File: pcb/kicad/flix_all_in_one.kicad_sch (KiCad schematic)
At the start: 0 parts

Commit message: Updated sch and added BoM.md
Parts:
- added U1: ESP32-WROOM-32E, RF_Module:ESP32-WROOM-32E, symbol RF_Module:ESP32-WROOM-32E
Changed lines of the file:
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@@
 	(generator_version "10.0")
 	(paper "A4")
+	(symbol
+		(lib_id "RF_Module:ESP32-WROOM-32E")
+		(at 148.59 102.87 0)
+		(unit 1)
+		(body_style 1)
+		(exclude_from_sim no)
+		(in_bom yes)
+		(on_board yes)
+		(in_pos_files yes)
+		(dnp no)
+		(fields_autoplaced yes)
+		(property "Reference" "U1"
+			(at 150.7333 64.77 0)
+			(show_name no)
+			(do_not_autoplace no)
+			(effects
+				(font
+					(size 1.27 1.27)
+				)
+				(justify left)
+			)
+		)
+		(property "Value" "ESP32-WROOM-32E"
+			(at 150.7333 67.31 0)
+			(show_name no)
+			(do_not_autoplace no)
+			(effects
+				(font
+					(size 1.27 1.27)
+				)
+				(justify left)
+			)
+		)
+		(property "Footprint" "RF_Module:ESP32-WROOM-32E"
+			(at 165.1 137.16 0)
+			(hide yes)
+			(show_name no)
+			(do_not_autoplace no)
+			(effects
+				(font
+					(size 1.27 1.27)
+				)
+			)
+		)
+		(property "Datasheet" "https://www.espressif.com/sites/default/files/documentation/esp32-wroom-32e_esp32-wroom-32ue_datasheet_en.pdf"
+			(at 148.59 102.87 0)
+			(hide yes)
+			(show_name no)
+			(do_not_autoplace no)
+			(effects
+				(font
+					(size 1.27 1.27)
+				)
+			)
+		)
+		(property "Description" "RF Module, ESP32-D0WD-V3 SoC, without PSRAM, Wi-Fi 802.11b/g/n, Bluetooth, BLE, 32-bit, 2.7-3.6V, onboard antenna, SMD"
+			(at 148.59 102.87 0)
+			(hide yes)
+			(show_name no)
+			(do_not_autoplace no)
+			(effects
+				(font
+					(size 1.27 1.27)
+				)
+			)
+		)
+		(pin "14"
+		)
+		(pin "11"
+		)
+		(pin "16"
+		)
+		(pin "12"
+		)
+		(pin "9"
+		)
+		(pin "17"
+		)
+		(pin "13"
+		)
+		(pin "30"
+		)
+		(pin "33"
+		)
+		(pin "27"
+		)
+		(pin "31"
+		)
+		(pin "10"
+		)
+		(pin "32"
+		)
+		(pin "34"
+		)
+		(pin "18"
+		)
+		(pin "26"
+		)
+		(pin "28"
+		)
+		(pin "19"
+		)
+		(pin "21"
+		)
+		(pin "35"
+		)
+		(pin "36"
+		)
+		(pin "29"
+		)
+		(pin "[1,15,38,39]"
+		)
+		(pin "3"
+		)
+		(pin "2"
+		)
+		(pin "20"
+		)
+		(pin "4"
+		)
+		(pin "25"
+		)
+		(pin "6"
+		)
+		(pin "24"
+		)
+		(pin "5"
+		)
+		(pin "7"
+		)
+		(pin "8"
+		)
+		(pin "37"
+		)
+		(pin "22"
+		)
+		(pin "23"
+		)
+		(instances
+			(project "flix_all_in_one"
+				(path "/b72e5080-03e0-4f53-a508-ed803e54cf11"
+					(reference "U1")
+					(unit 1)
+				)
+			)
+		)
+	)
 	(sheet_instances
 		(path "/"

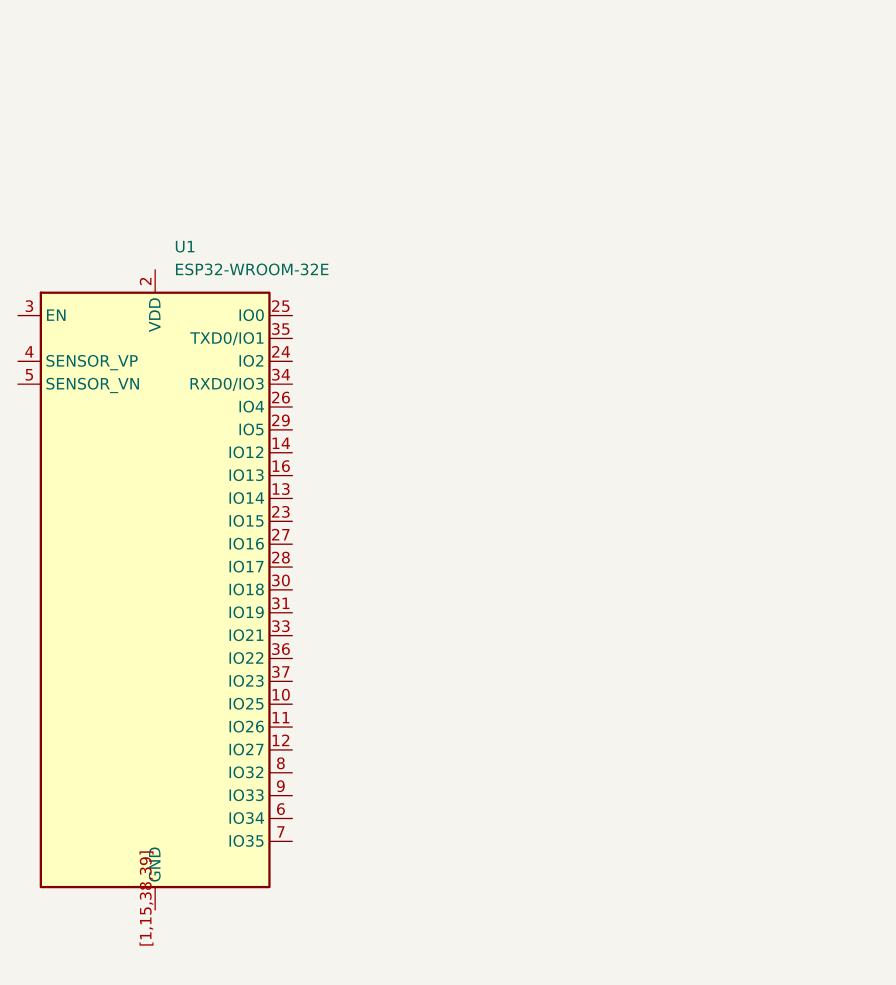
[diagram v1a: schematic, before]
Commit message: .
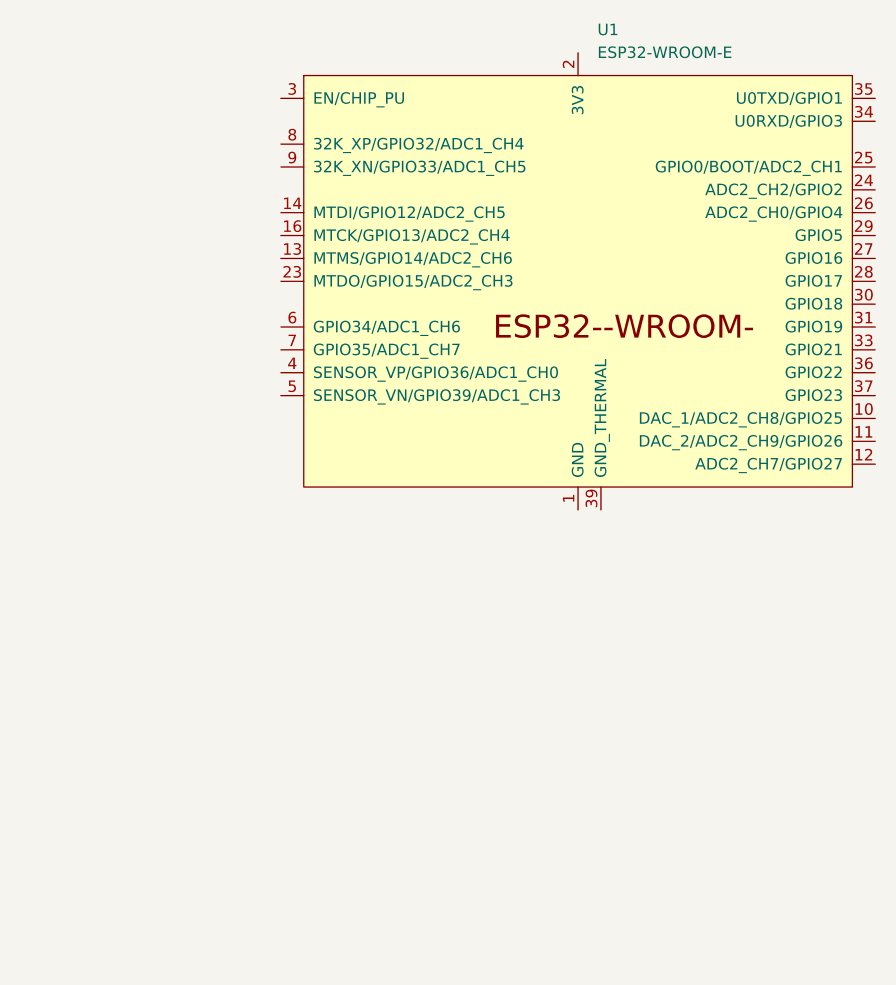
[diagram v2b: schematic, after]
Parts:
- removed U1: ESP32-WROOM-32E, RF_Module:ESP32-WROOM-32E, symbol RF_Module:ESP32-WROOM-32E
- added U1: ESP32-WROOM-E, PCM_Espressif:ESP32-WROOM-32E, symbol PCM_Espressif:ESP32-WROOM-E
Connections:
- new net: U1.1 (GND), U1.15 (GND), U1.38 (GND)
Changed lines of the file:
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@@
 	(paper "A4")
 	(symbol
-		(lib_id "RF_Module:ESP32-WROOM-32E")
-		(at 148.59 102.87 0)
+		(lib_id "PCM_Espressif:ESP32-WROOM-E")
+		(at 195.58 68.58 0)
 		(unit 1)
 		(body_style 1)
@@
 		(fields_autoplaced yes)
 		(property "Reference" "U1"
-			(at 150.7333 64.77 0)
+			(at 197.7233 40.64 0)
 			(show_name no)
 			(do_not_autoplace no)
@@
 			)
 		)
-		(property "Value" "ESP32-WROOM-32E"
-			(at 150.7333 67.31 0)
+		(property "Value" "ESP32-WROOM-E"
+			(at 197.7233 43.18 0)
 			(show_name no)
 			(do_not_autoplace no)
@@
 			)
 		)
-		(property "Footprint" "RF_Module:ESP32-WROOM-32E"
-			(at 165.1 137.16 0)
+		(property "Footprint" "PCM_Espressif:ESP32-WROOM-32E"
+			(at 195.58 104.14 0)
 			(hide yes)
 			(show_name no)
@@
 		)
 		(property "Datasheet" "https://www.espressif.com/sites/default/files/documentation/esp32-wroom-32e_esp32-wroom-32ue_datasheet_en.pdf"
-			(at 148.59 102.87 0)
+			(at 195.58 106.68 0)
 			(hide yes)
 			(show_name no)
@@
 			)
 		)
-		(property "Description" "RF Module, ESP32-D0WD-V3 SoC, without PSRAM, Wi-Fi 802.11b/g/n, Bluetooth, BLE, 32-bit, 2.7-3.6V, onboard antenna, SMD"
-			(at 148.59 102.87 0)
+		(property "Description" "ESP32-WROOM-32E integrates ESP32-D0WD-V3, with higher stability and safety performance."
+			(at 195.58 68.58 0)
 			(hide yes)
 			(show_name no)
@@
 			)
 		)
-		(pin "14"
+		(pin "15"
 		)
-		(pin "11"
+		(pin "30"
 		)
-		(pin "16"
-		)
-		(pin "12"
-		)
-		(pin "9"
-		)
-		(pin "17"
+		(pin "31"
 		)
 		(pin "13"
 		)
-		(pin "30"
-		)
-		(pin "33"
-		)
-		(pin "27"
-		)
-		(pin "31"
-		)
-		(pin "10"
-		)
-		(pin "32"
-		)
-		(pin "34"
-		)
-		(pin "18"
-		)
-		(pin "26"
-		)
-		(pin "28"
-		)
-		(pin "19"
-		)
-		(pin "21"
+		(pin "25"
 		)
 		(pin "35"
@@
 		(pin "36"
 		)
+		(pin "33"
+		)
 		(pin "29"
 		)
-		(pin "[1,15,38,39]"
+		(pin "34"
+		)
+		(pin "37"
+		)
+		(pin "14"
+		)
+		(pin "7"
+		)
+		(pin "26"
+		)
+		(pin "9"
+		)
+		(pin "27"
+		)
+		(pin "5"
+		)
+		(pin "4"
 		)
 		(pin "3"
 		)
-		(pin "2"
+		(pin "23"
 		)
-		(pin "20"
+		(pin "39"
 		)
-		(pin "4"
+		(pin "12"
 		)
-		(pin "25"
+		(pin "28"
+		)
+		(pin "16"
+		)
+		(pin "38"
+		)
+		(pin "11"
+		)
+		(pin "8"
+		)
+		(pin "10"
 		)
 		(pin "6"
 		)
+		(pin "2"
+		)
+		(pin "1"
+		)
 		(pin "24"
 		)
-		(pin "5"
-		)
-		(pin "7"
-		)
-		(pin "8"
-		)
-		(pin "37"
-		)
-		(pin "22"
-		)
-		(pin "23"
-		)
 		(instances
